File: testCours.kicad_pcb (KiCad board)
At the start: 2 copper layers, 68.6 x 53.3 mm, 21 parts, among them P1 Power, P2 Analog, P3 Digital, P4 Digital, P5 CONN_01X01, P6 CONN_01X01, P7 CONN_01X01, P8 CONN_01X01, U1 RN2483BREAKOUT, U2 LTC1050

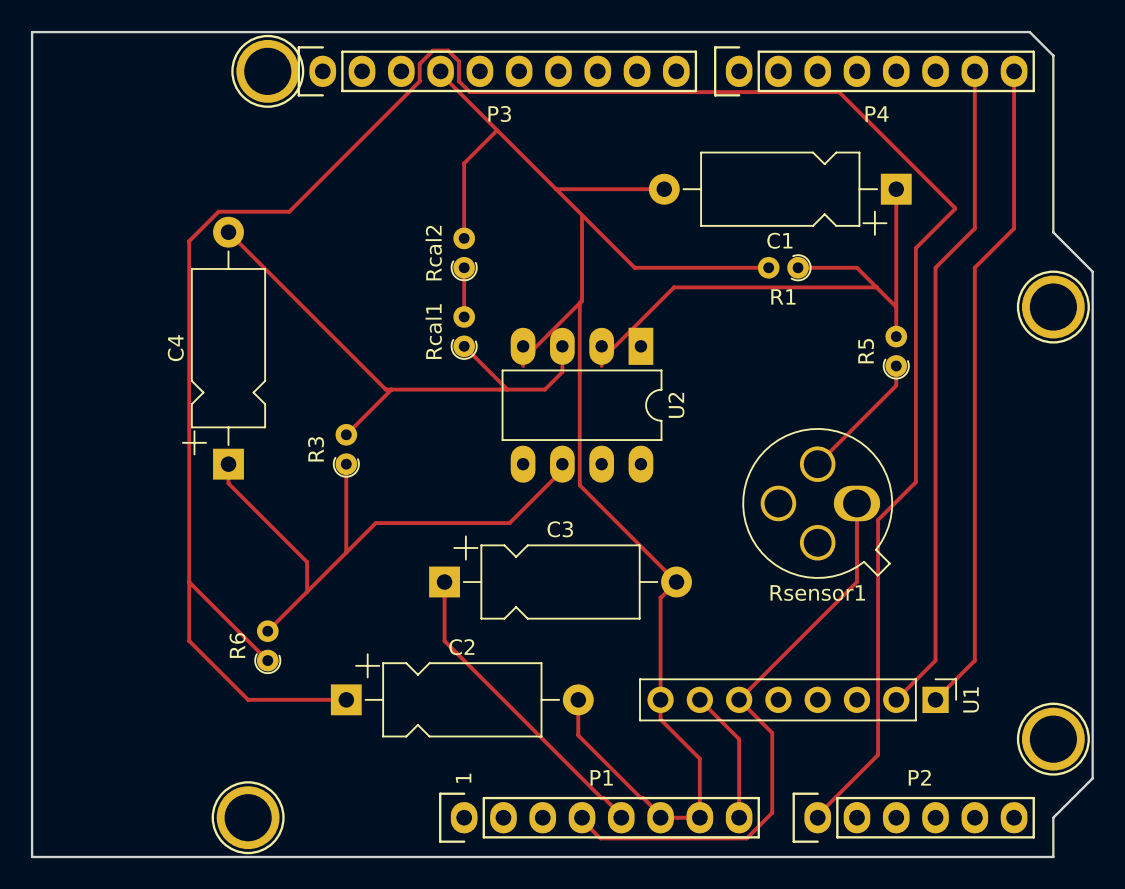
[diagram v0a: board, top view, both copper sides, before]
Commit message: fin
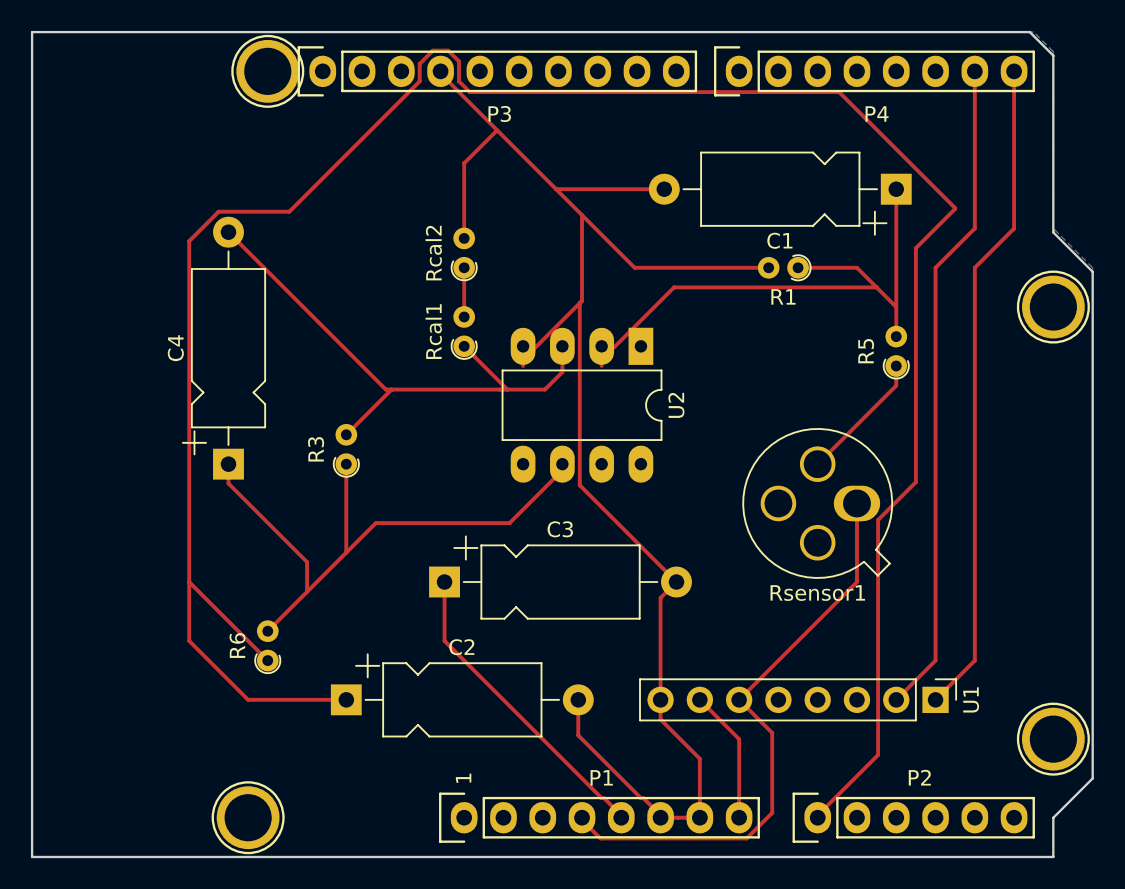
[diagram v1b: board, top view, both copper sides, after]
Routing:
- added copper zone on B.Cu, net (none)
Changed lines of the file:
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@@
   (segment (start 161.798 100.965) (end 166.878 95.885) (width 0.25) (layer F.Cu) (net 39))
   (segment (start 138.938 91.445) (end 138.938 88.265) (width 0.25) (layer F.Cu) (net 43))
+  (zone (net 0) (net_name "") (layer B.Cu) (hatch edge 0.508)
+    (connect_pads (clearance 0.508))
+    (min_thickness 0.254)
+    (fill yes (arc_segments 16) (thermal_gap 0.508) (thermal_bridge_width 0.508))
+    (polygon
+      (pts
+        (xy 110.998 73.025) (xy 110.998 126.365) (xy 177.038 126.365) (xy 177.038 123.825) (xy 179.578 121.285)
+        (xy 179.578 88.265) (xy 177.038 85.725) (xy 177.038 74.295) (xy 175.768 73.025)
+      )
+    )
+  )
 )
